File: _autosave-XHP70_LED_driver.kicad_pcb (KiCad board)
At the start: 2 copper layers, 17 x 17 mm, 24 parts, among them U1 TPS61088, U2 ATtiny816_(QFN20), U3 INA181

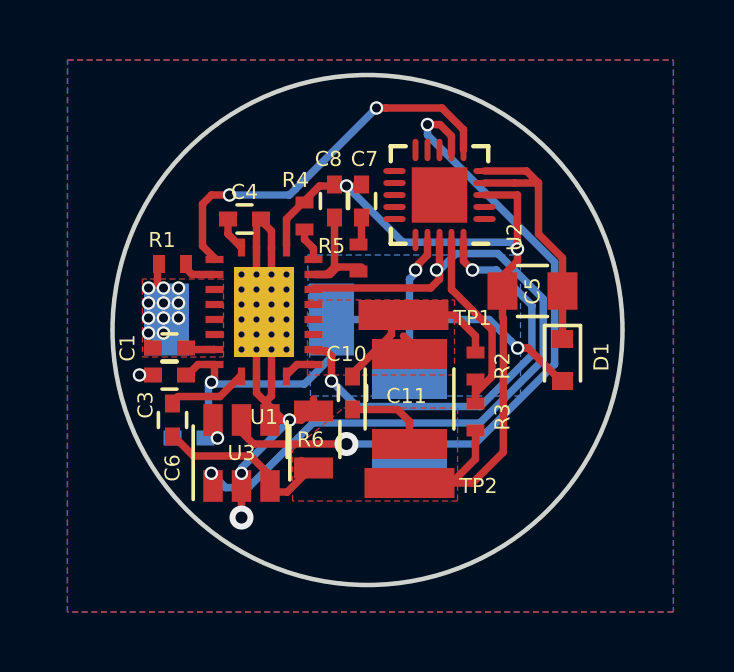
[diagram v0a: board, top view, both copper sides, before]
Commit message: finished, ready for prod.
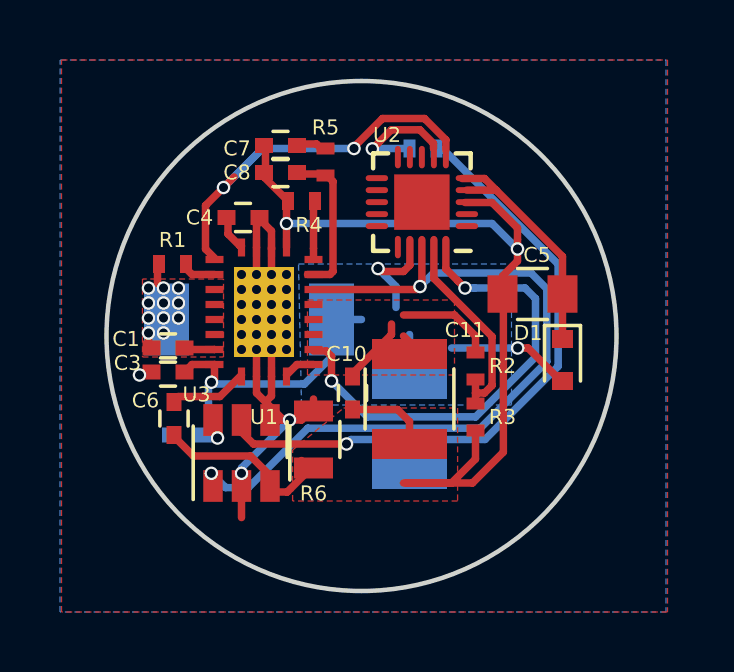
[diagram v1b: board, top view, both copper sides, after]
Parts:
- removed TP1, TP2: TestPoint, Misc:flashlight_batt
- added R7: 100k, Resistors_SMD:R_0402_NoSilk, B.Cu at (105.0, 51.5)
- C7: value C -> 3.3nF
- C8: value C -> 100pF
- moved R5 3.38 mm to (101.8, 52.0)
- moved C7 3.27 mm to (100.3, 51.5), turned to 0 degrees
- moved C8 2.04 mm to (100.3, 52.4), turned to 0 degrees
- moved U2 0.63 mm to (105.0, 53.3)
- moved R4 0.51 mm to (101.0, 53.3), turned to 0 degrees
- moved C3 0.11 mm to (96.5, 59.0)
- moved C9 0.11 mm to (97.2, 61.1)
- moved C5 0.10 mm to (108.7, 56.4)
- moved C6 0.07 mm to (96.8, 60.5)
- moved C4 0.07 mm to (99.0, 53.9)
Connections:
- U3 pad 5: /DAC_OUT -> Net-(R7-Pad2)
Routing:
- net Net-(R7-Pad2): track 0.00 -> 21.2 mm, vias 0 -> 1
- net /DAC_OUT: track 23.4 -> 3.96 mm, vias 2 -> 1
- net +BATT: track 23.6 -> 20.9 mm
- net /MODE: track 14.5 -> 15.9 mm
- net /LED_K: track 36.6 -> 38.0 mm
- net Net-(C8-Pad2): track 4.01 -> 5.19 mm
- net Net-(C5-Pad2): track 9.20 -> 8.07 mm
- net Net-(R4-Pad2): track 1.17 -> 1.95 mm
- net /ENABLE: track 13.0 -> 13.8 mm
- net GND: vias 4 -> 3
